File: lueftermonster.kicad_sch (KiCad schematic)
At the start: 94 parts, among them J1 Barrel_Jack, J10 Fan, J11 Fan, J12 Fan, J13 Fan, J14 Fan, J15 Fan, J16 Fan, J17 PROG, J2 Fan, J3 Fan, J4 Fan, J5 Fan, J6 Fan, J7 Fan, J8 Fan, J9 Fan, Q1 Q_PMOS_GSD, Q2 Q_NMOS_GSD, Q3 Q_NMOS_GSD, Q4 Q_NMOS_GSD, Q5 Q_NMOS_GSD, U1 ESP32-WROOM-32E, U2 AOZ1280CI, U3 AMS1117-5.0

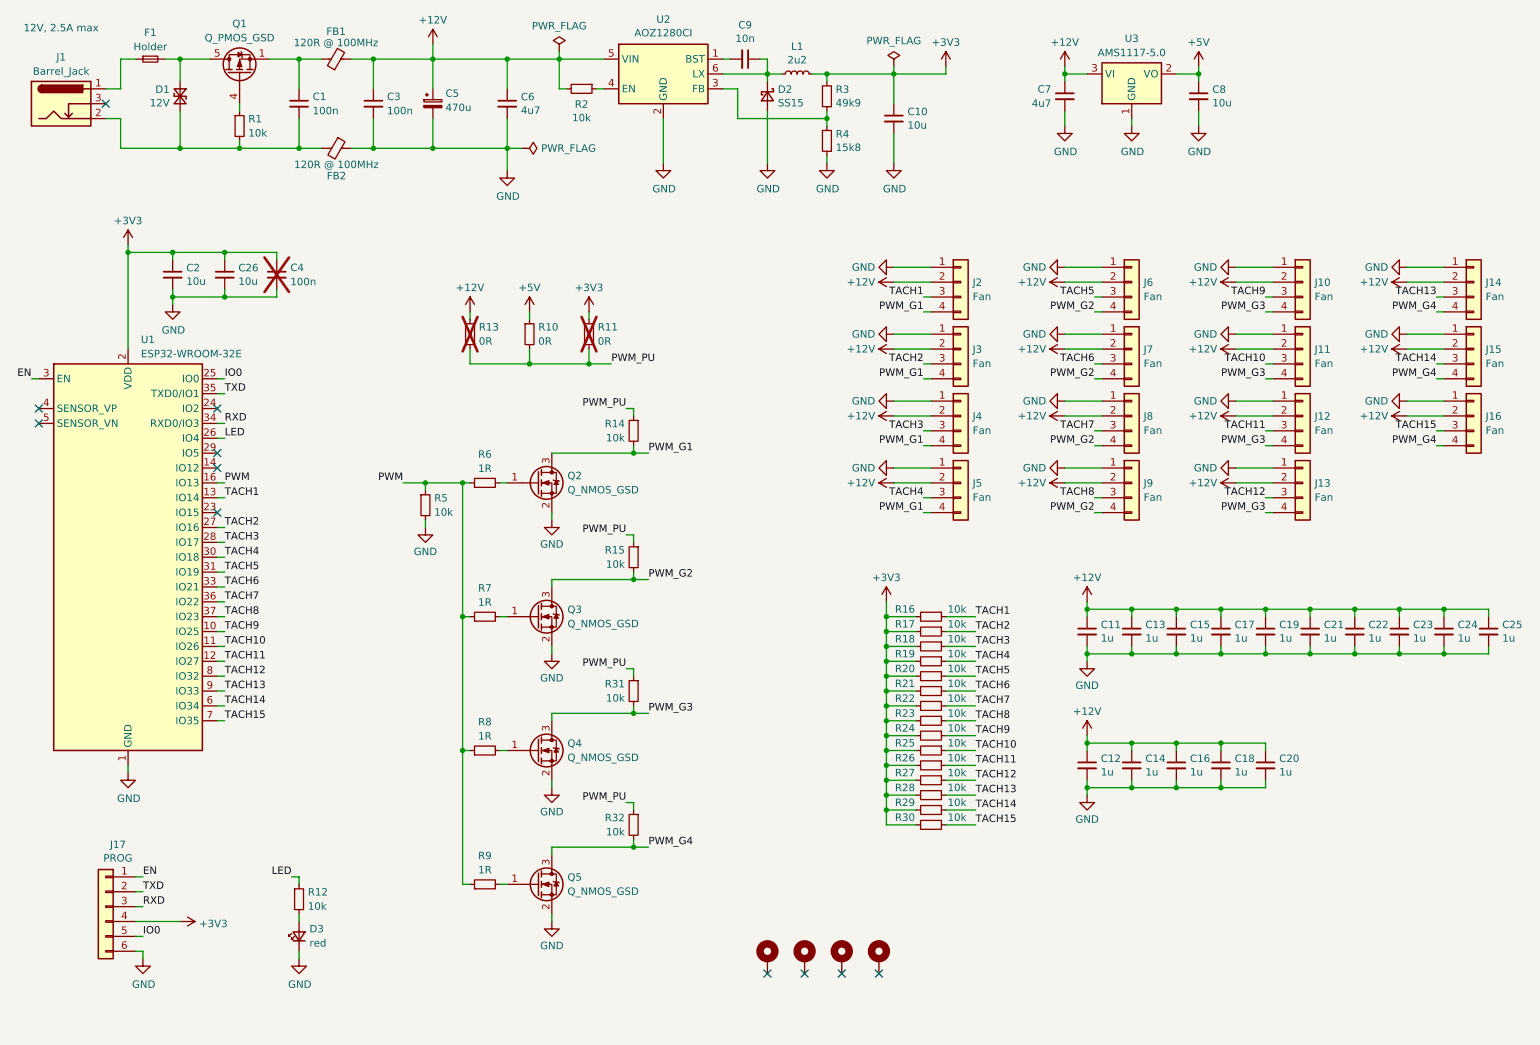
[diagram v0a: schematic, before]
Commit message: snap
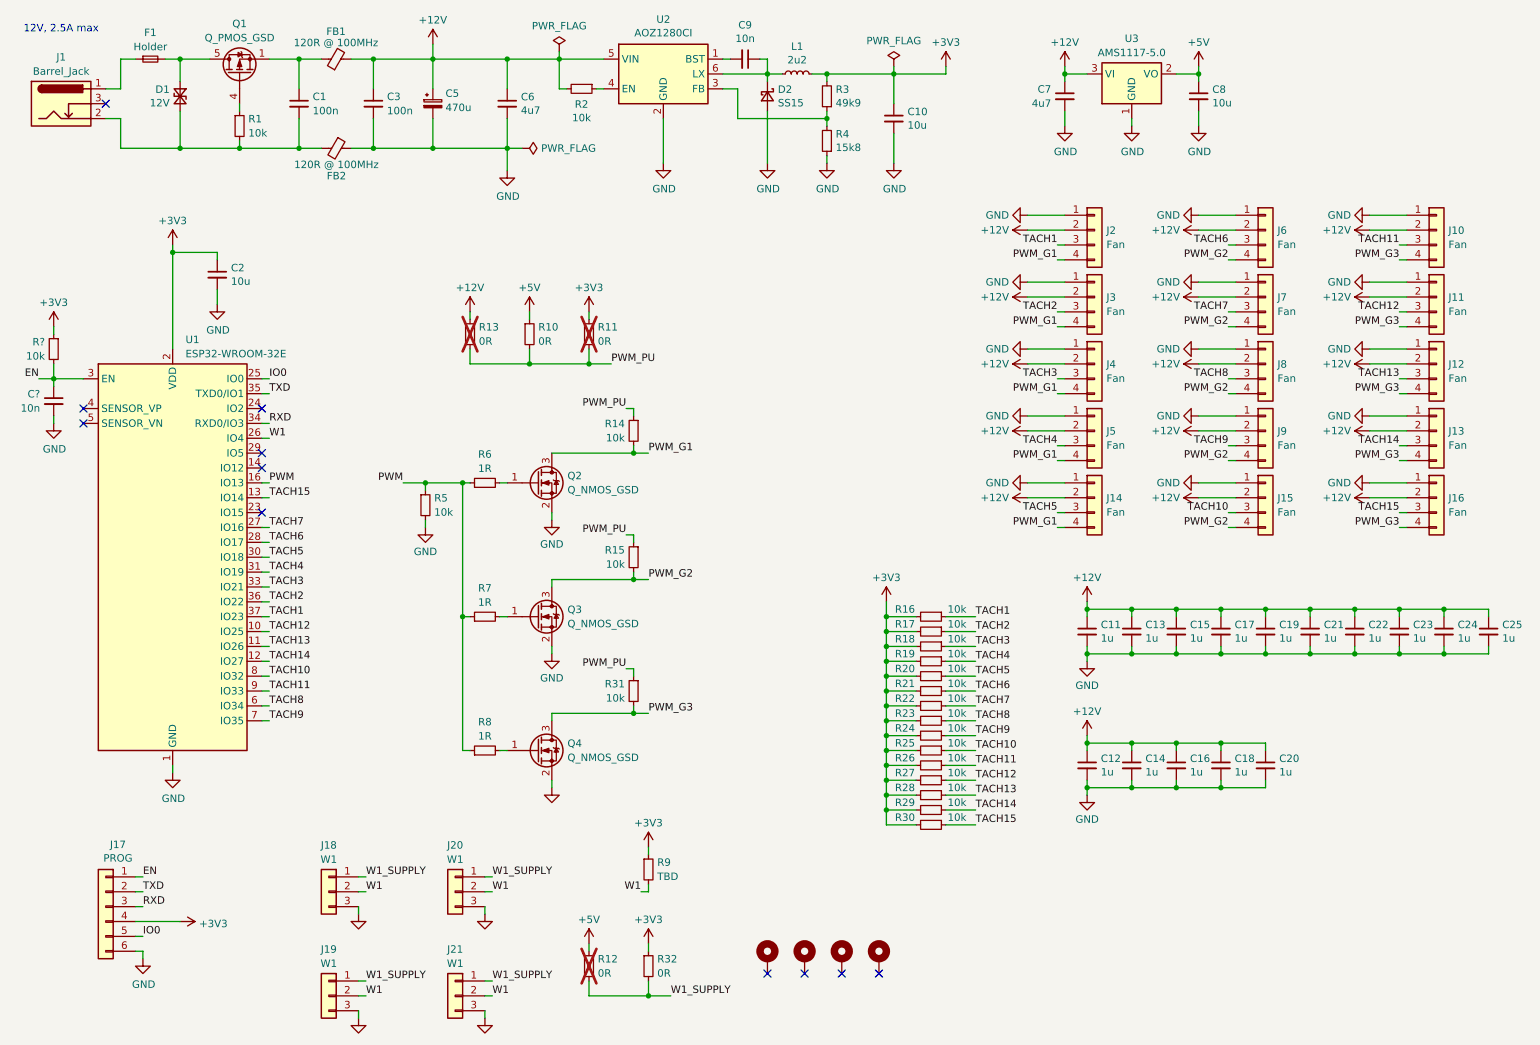
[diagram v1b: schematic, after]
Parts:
- removed C26: 10u, Capacitor_SMD:C_0805_2012Metric, symbol Device:C_Small
- removed C4: 100n, Capacitor_SMD:C_0402_1005Metric, symbol Device:C_Small
- removed D3: red, LED_SMD:LED_0603_1608Metric, symbol Device:LED_Small
- removed Q5: Q_NMOS_GSD, Package_TO_SOT_SMD:SOT-23, symbol Device:Q_NMOS_GSD
- added C?: 10n, Capacitor_SMD:C_0402_1005Metric, symbol Device:C_Small
- added J18, J19, J20, J21: W1, Connector_PinHeader_2.54mm:PinHeader_1x03_P2.54mm_Vertical_SMD_Pin1Left, symbol Connector_Generic:Conn_01x03
- added R?: 10k, Resistor_SMD:R_0402_1005Metric, symbol Device:R_Small
- L1: footprint Inductor_SMD:L_Taiyo-Yuden_NR-24xx -> Inductor_SMD:L_1008_2520Metric; Digikey 587-3443-1-ND -> (none); LCSC (none) -> C576403; MPN NRH2412T2R2MNGH -> DFE252012F-2R2M=P2; Manufacturer Taiyo Yuden -> Murata Electronics
- R12: value 10k -> 0R; footprint Resistor_SMD:R_0402_1005Metric -> Resistor_SMD:R_0603_1608Metric_Pad0.98x0.95mm_HandSolder; LCSC C25744 -> C21189; MPN 0402WGF1002TCE -> 0603WAF0000T5E; now not fitted
- R32: value 10k -> 0R; footprint Resistor_SMD:R_0402_1005Metric -> Resistor_SMD:R_0603_1608Metric_Pad0.98x0.95mm_HandSolder; LCSC C25744 -> C21189; MPN 0402WGF1002TCE -> 0603WAF0000T5E
- R9: value 1R -> TBD; LCSC C25086 -> (none); MPN 0402WGF100KTCE -> (none); Manufacturer UNI-ROYAL(Uniroyal Elec) -> (none)
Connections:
- net +3V3: now also R32.1, R9.1, R?.1
- net +5V: now also R12.1
- net EN: now also C?.1, R?.2
- net GND: now also C?.2, J18.3 (Pin_3), J19.3 (Pin_3), J20.3 (Pin_3), J21.3 (Pin_3)
- net PWM: no longer R9.1
- net PWM_G1: now also J14.4 (Pin_4)
- net PWM_G2: now also J15.4 (Pin_4)
- net PWM_G3: now also J16.4 (Pin_4)
- net PWM_PU: no longer R32.1
- net TACH1: now also U1.37 (IO23); no longer U1.13 (IO14)
- net TACH10: now also J15.3 (Pin_3), U1.8 (IO32); no longer J11.3 (Pin_3), U1.11 (IO26)
- net TACH11: now also J10.3 (Pin_3), U1.9 (IO33); no longer J12.3 (Pin_3), U1.12 (IO27)
- net TACH12: now also J11.3 (Pin_3), U1.10 (IO25); no longer J13.3 (Pin_3), U1.8 (IO32)
- net TACH13: now also J12.3 (Pin_3), U1.11 (IO26); no longer J14.3 (Pin_3), U1.9 (IO33)
- net TACH14: now also J13.3 (Pin_3), U1.12 (IO27); no longer J15.3 (Pin_3), U1.6 (IO34)
- net TACH15: now also U1.13 (IO14); no longer U1.7 (IO35)
- net TACH2: now also U1.36 (IO22); no longer U1.27 (IO16)
- net TACH3: now also U1.33 (IO21); no longer U1.28 (IO17)
- net TACH4: now also U1.31 (IO19); no longer U1.30 (IO18)
- net TACH5: now also J14.3 (Pin_3), U1.30 (IO18); no longer J6.3 (Pin_3), U1.31 (IO19)
- net TACH6: now also J6.3 (Pin_3), U1.28 (IO17); no longer J7.3 (Pin_3), U1.33 (IO21)
- net TACH7: now also J7.3 (Pin_3), U1.27 (IO16); no longer J8.3 (Pin_3), U1.36 (IO22)
- net TACH8: now also J8.3 (Pin_3), U1.6 (IO34); no longer J9.3 (Pin_3), U1.37 (IO23)
- net TACH9: now also J9.3 (Pin_3), U1.7 (IO35); no longer J10.3 (Pin_3), U1.10 (IO25)
- net W1_SUPPLY: now reaches R12.2
- net W1_SUPPLY: now also R32.2, J18.1 (Pin_1), J19.1 (Pin_1), J20.1 (Pin_1), J21.1 (Pin_1)
- net W1: now reaches R9.2
- net W1: now also U1.26 (IO4), J18.2 (Pin_2), J19.2 (Pin_2), J20.2 (Pin_2), J21.2 (Pin_2)
- removed net LED: R12.1, U1.26 (IO4)
- removed net PWM_G4: J14.4 (Pin_4), J15.4 (Pin_4), J16.4 (Pin_4), R32.2
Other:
- moved on the sheet: C2, J10, J11, J12, J13, J14, J15, J16, J2, J3, J4, J5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
